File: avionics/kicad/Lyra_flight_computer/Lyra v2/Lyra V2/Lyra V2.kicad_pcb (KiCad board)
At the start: 4 copper layers, 40 x 75 mm, 90 parts, among them J1 USB_B_Micro, J10 Conn_01x04, J11 Conn_01x04, J12 Conn_01x03, J13 MEM2067-02-180-00-A, J2 Screw_Terminal_01x04, J3 Screw_Terminal_01x04, J4 Conn_02x03_Odd_Even, J5 Screw_Terminal_01x04, J6 Screw_Terminal_01x04, J7 Conn_02x03_Odd_Even, J8 Conn_02x03_Odd_Even, J9 Conn_02x03_Odd_Even, Q1 AO3401A, Q2 BSS138, Q3 BSS138, SW1 SW_Push_DPDT, U1 AZ1117-3.3, U2 AZ1117-5.0, U3 LIS3MDL, U4 BMP390L, U5 W25Q128JVS, U6 RP2040, U7 BMI088, X1 ECS-2520MV-xxx-xx

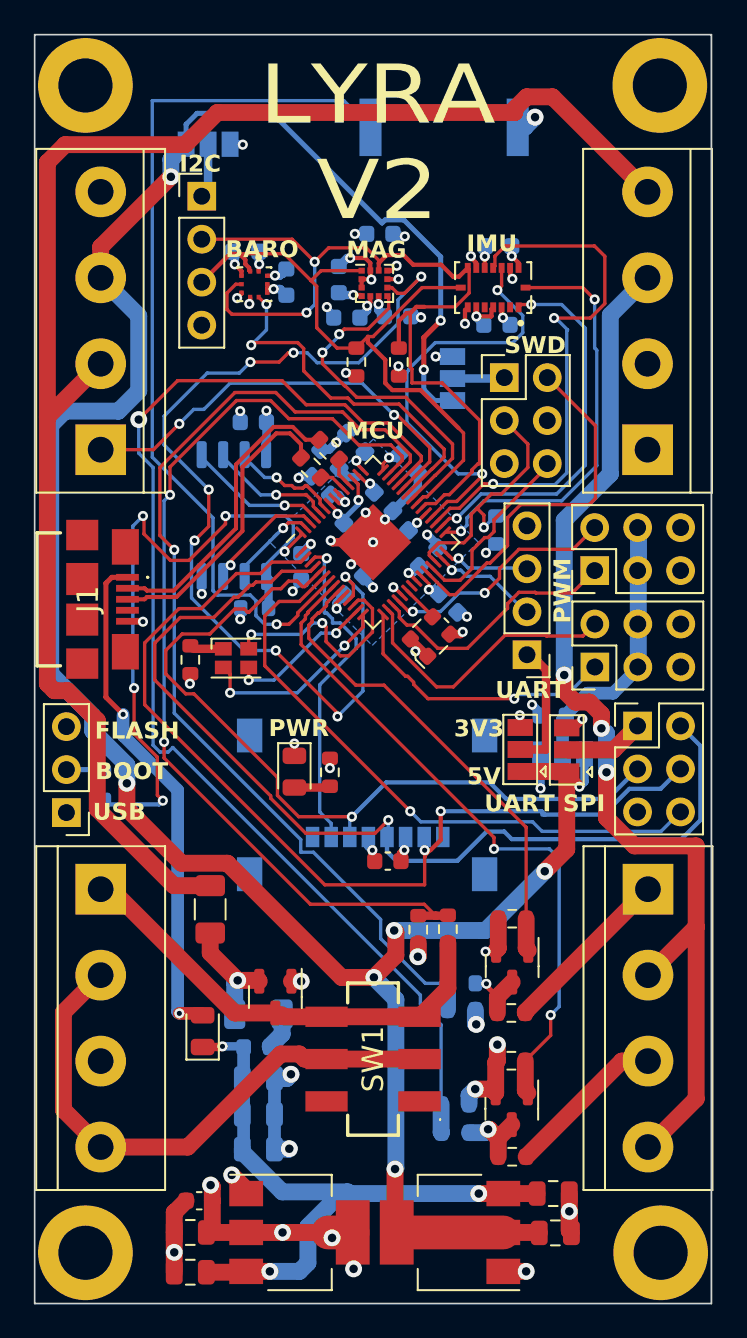
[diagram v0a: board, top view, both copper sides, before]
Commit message: lots of things
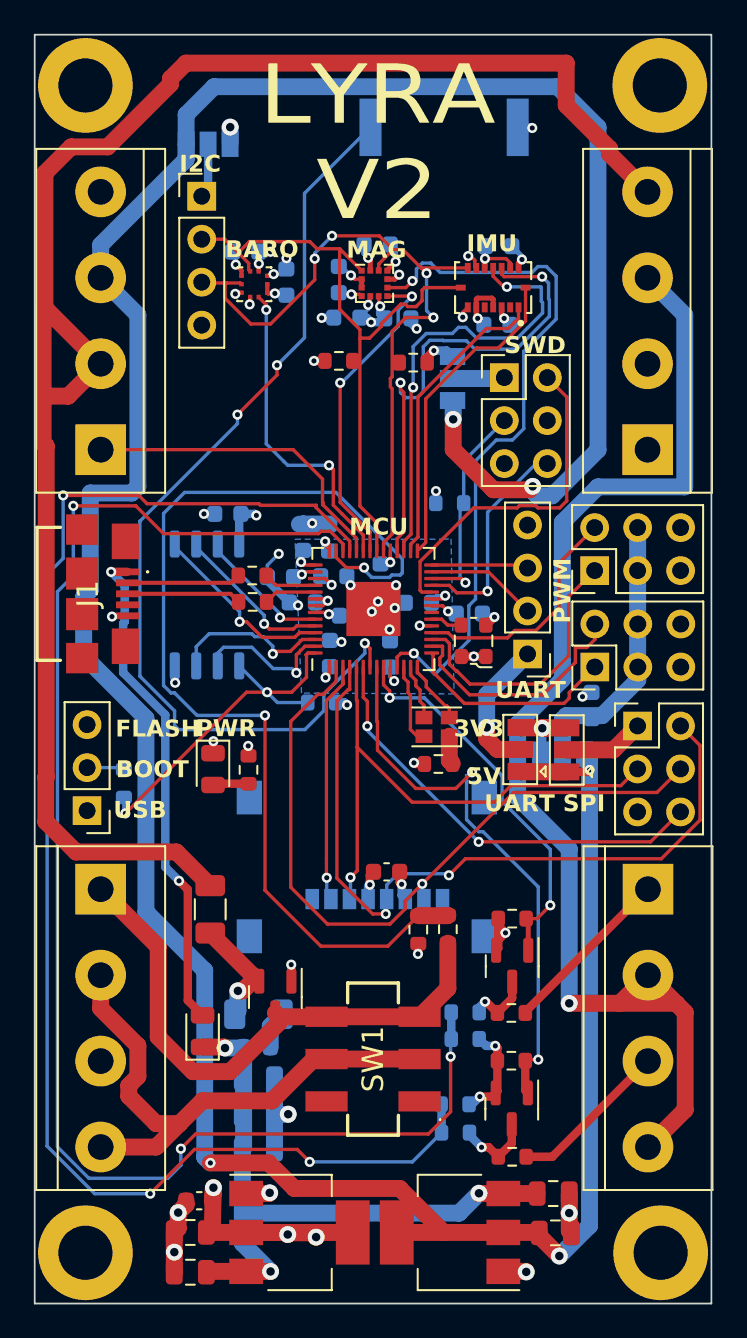
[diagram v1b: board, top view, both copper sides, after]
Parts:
- moved R12 15.9 mm to (123.8, 105.3), turned to 180 degrees
- moved D3 12.5 mm to (123.7, 103.1), turned to 180 degrees
- moved C27 9.97 mm to (115.7, 95.7), turned to 180 degrees
- moved C23 9.57 mm to (125.6, 96.4), turned to 0 degrees
- moved R16 8.72 mm to (112.8, 94.1), turned to 180 degrees
- moved R15 8.65 mm to (112.8, 95.7), turned to 0 degrees
- moved C30 8.15 mm to (117.3, 98.7), turned to 90 degrees
- moved C21 7.55 mm to (114.4, 94.2), turned to 180 degrees
- moved C20 6.94 mm to (117.6, 94.2), turned to 0 degrees
- moved R14 6.84 mm to (116.9, 101.6), turned to 180 degrees
- moved C15 5.70 mm to (118.7, 96.5), turned to 0 degrees
- moved C17 5.67 mm to (122.6, 95.7), turned to 180 degrees
- moved C18 5.63 mm to (111.3, 90.5)
- moved U5 5.52 mm to (110.1, 95.9)
- moved D2 4.81 mm to (110.4, 105.6)
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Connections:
- net Net-(U6-USB_DM) renamed /RP USB_D-
- net Net-(U6-USB_DP) renamed /RP USB_D+
- J10 pad 2: /I2C1 SDA -> /I2C1 SCL
- J10 pad 3: /I2C1 SCL -> /I2C1 SDA
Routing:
- net +5V: track 147.5 -> 190.5 mm, vias 9 -> 5
- net /P1 CONT: track 60.4 -> 87.8 mm, vias 1 -> 3
- net /QSPI_SS: track 40.9 -> 21.9 mm, vias 5 -> 2
- net /SPI0 MISO: track 58.0 -> 42.3 mm, vias 2 -> 1
- net /SPI0 MOSI: track 48.1 -> 32.6 mm
- net /MAG DRDY: track 57.4 -> 42.1 mm, vias 8 -> 2
- net /SPI0 SCLK: track 59.6 -> 44.6 mm, vias 1 -> 2
- net /P2 CONT: track 72.1 -> 85.8 mm, vias 1 -> 3
- net GND: track 70.6 -> 58.9 mm, vias 44 -> 41
- net /USB_D-: track 17.9 -> 6.73 mm
- net /USB_D+: track 17.6 -> 6.77 mm
- net /BRKOUT CS: track 36.6 -> 25.8 mm, vias 1 -> 2
- net /I2C1 SDA: track 52.8 -> 43.0 mm, vias 2 -> 4
- net +12P: track 92.4 -> 101.9 mm
- net /PYRO PWR: track 64.5 -> 72.9 mm, vias 3 -> 1
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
